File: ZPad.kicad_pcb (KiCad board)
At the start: 2 copper layers, 83.5 x 69 mm, 19 parts, among them J1 Conn_01x04, SW1 SW_Push, SW2 SW_Push, SW3 SW_Push, SW4 SW_Push, SW5 SW_Push, SW6 SW_Push, SW7 SW_Push, SW8 SW_Push, SW9 RotaryEncoder_Switch, U1 MOUDLE-SEEEDUINO-XIAO

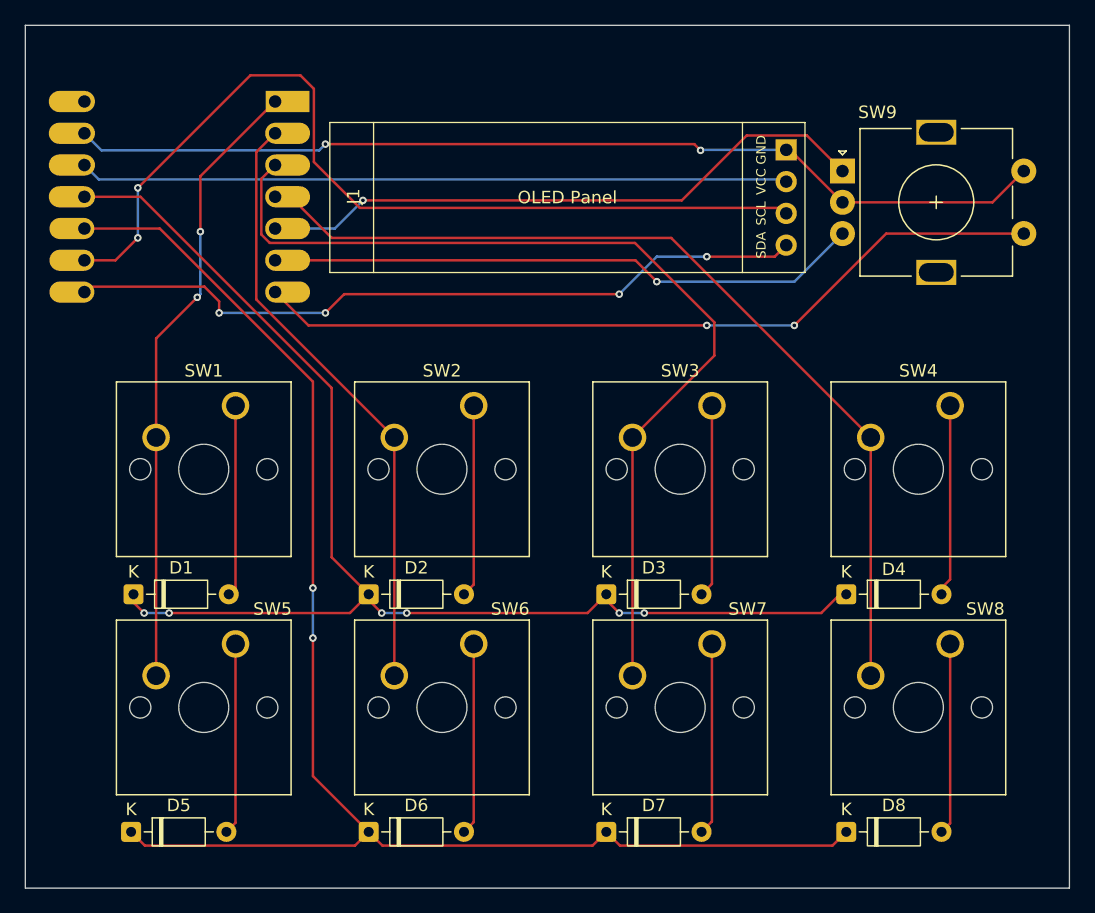
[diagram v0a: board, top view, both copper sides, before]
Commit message: Routed PCB again cuz XIAO was flipped
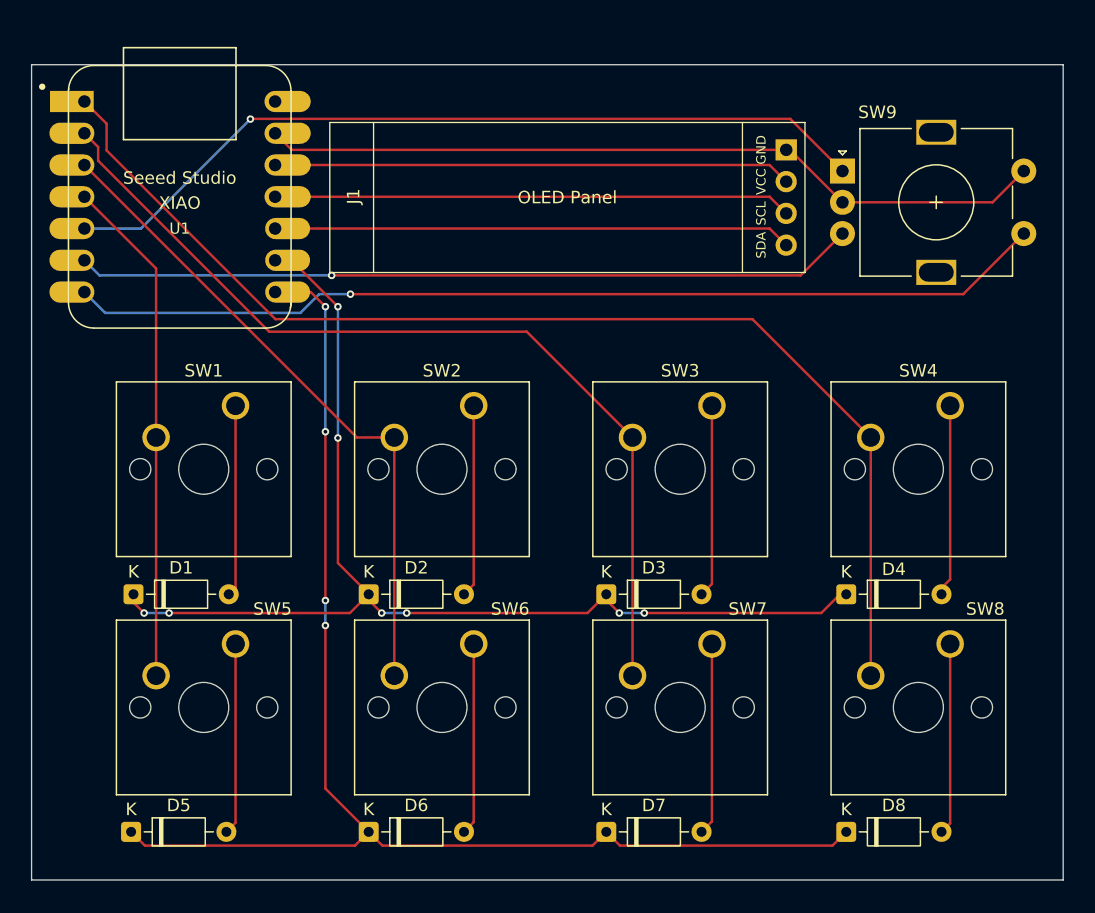
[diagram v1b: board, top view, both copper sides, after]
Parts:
- U1: moved to F.Cu
- turned U1 to 0 degrees
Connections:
- U1 pad 1: /COL0 -> /COL3
- U1 pad 10: /ROW1 -> /SDA
- U1 pad 11: /ROW0 -> /SCL
- U1 pad 2: /COL1 -> /COL2
- U1 pad 3: /COL2 -> /COL1
- U1 pad 4: /COL3 -> /COL0
- U1 pad 8: /SDA -> /ROW1
- U1 pad 9: /SCL -> /ROW0
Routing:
- net /SCL: track 72.6 -> 42.5 mm, vias 2 -> 0
- net /COL3: track 75.7 -> 94.3 mm
- net /SDA: track 60.0 -> 41.4 mm, vias 4 -> 0
- net /Rotary_Sw_A: track 49.6 -> 66.0 mm
- net GND: track 78.9 -> 63.2 mm, vias 2 -> 0
- net +3V3: track 56.7 -> 41.4 mm
- net /Rotary_Sw_B: track 47.7 -> 62.5 mm
- net /Rotary_Sw_S1: track 64.0 -> 78.4 mm, vias 2 -> 1
- net /ROW1: track 121.1 -> 107.9 mm, vias 2 -> 4
- net /ROW0: track 105.7 -> 92.4 mm, vias 6 -> 8
- net /COL0: track 49.9 -> 40.7 mm, vias 2 -> 0
- net /COL1: track 48.6 -> 52.9 mm
- net /COL2: track 76.1 -> 73.6 mm
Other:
- board size 83.5 x 69 mm -> 82.5 x 65.2 mm
